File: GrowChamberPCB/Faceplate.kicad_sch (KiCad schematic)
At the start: 34 parts, among them J1 Conn_01x02_Pin, J10 Conn_01x02_Pin, J11 Conn_01x02_Pin, J12 Conn_01x03_Pin, J13 Conn_01x03_Pin, J14 Conn_01x03_Pin, J15 Conn_01x04_Pin, J2 Conn_01x03_Pin, J3 Conn_01x04_Pin, J4 Conn_01x02_Pin, J5 Conn_01x02_Pin, J6 Conn_01x02_Pin, J7 Conn_01x02_Pin, J8 Conn_01x02_Pin, J9 Conn_01x02_Pin, SW2 ResetButton_External, SW4 BootMode_External, U19 To Faceplate, U20 PCA9555APW,118

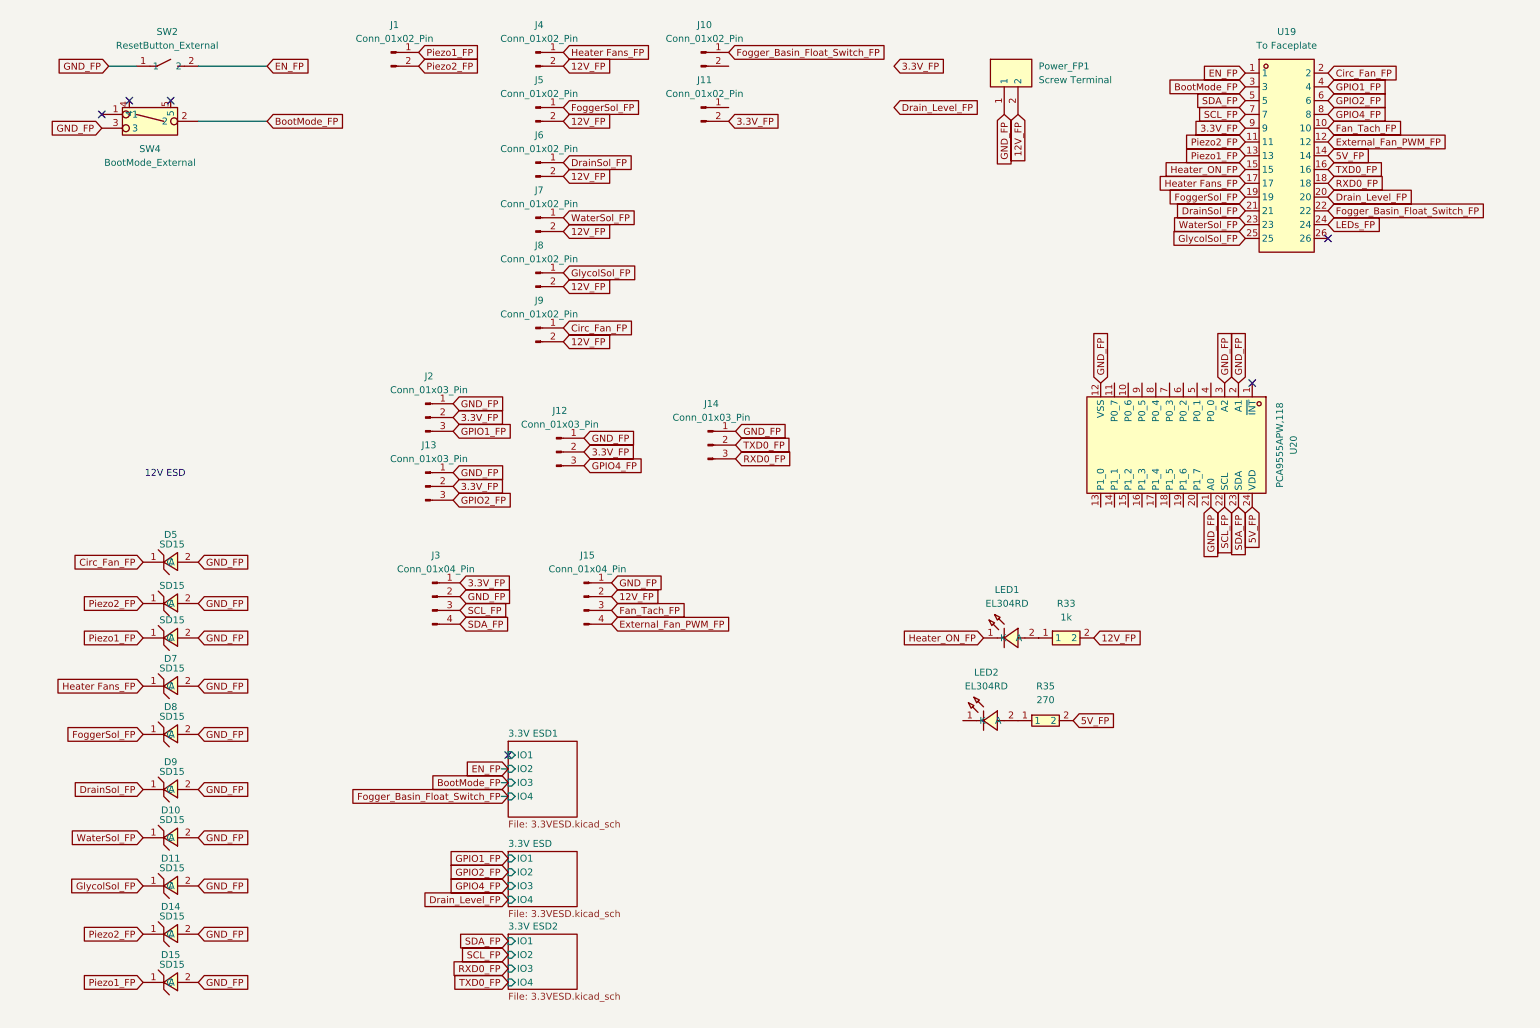
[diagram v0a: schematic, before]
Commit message: started PCB
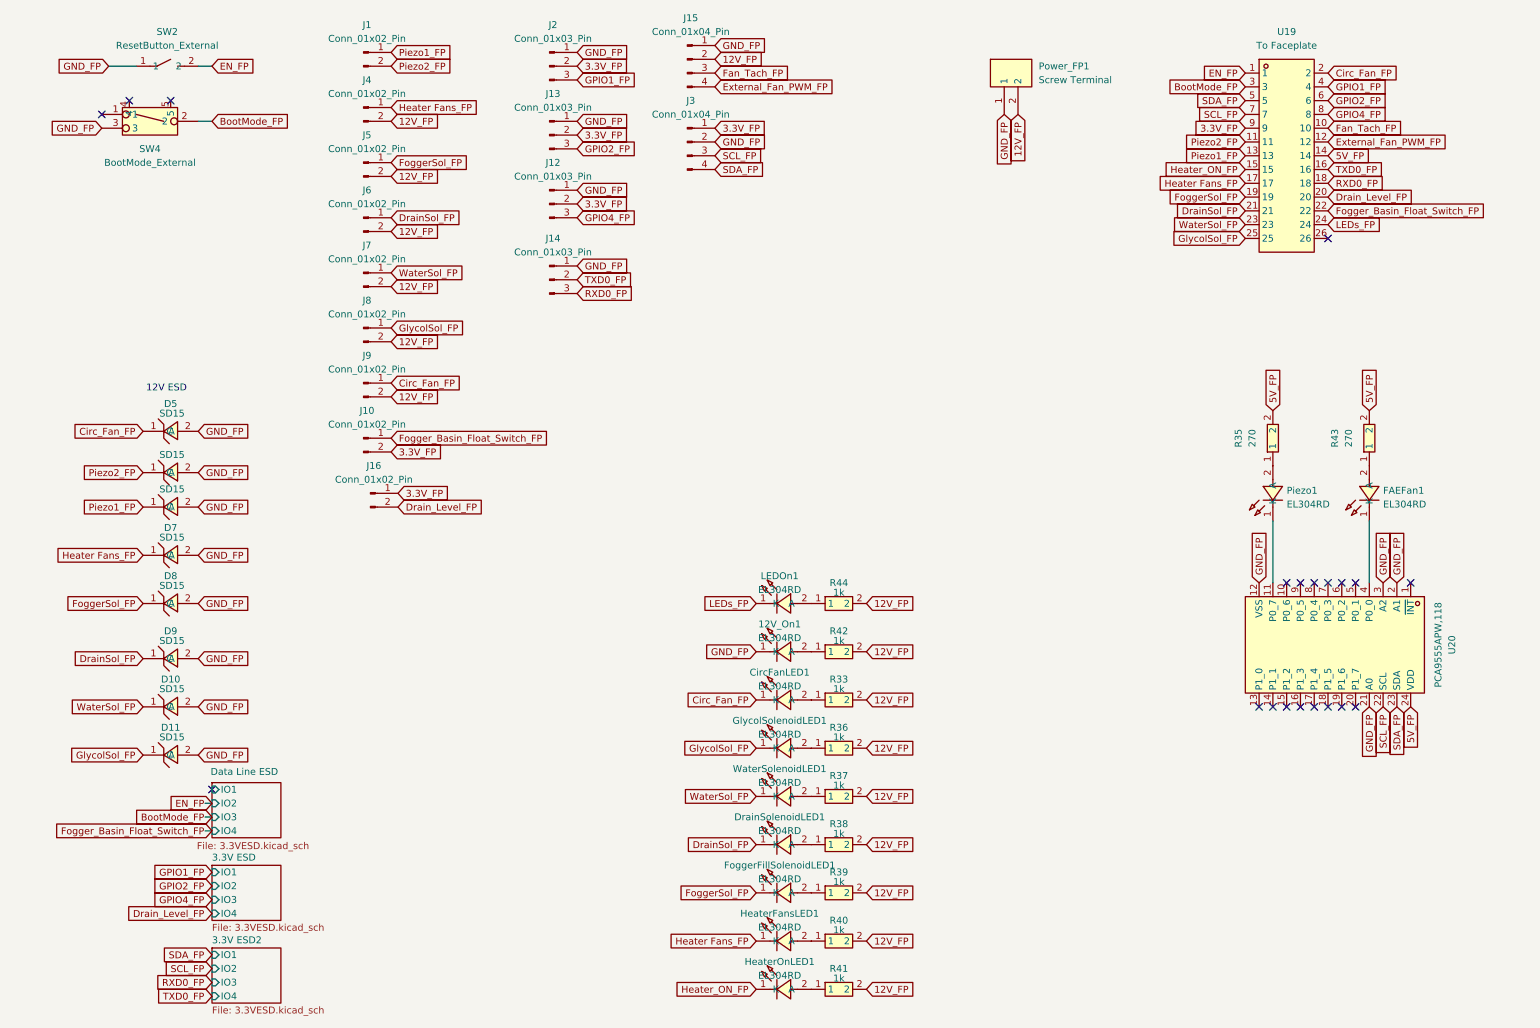
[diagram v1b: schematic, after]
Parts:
- removed D14, D15: SD15, easyeda2kicad:SOD-323_L1.7-W1.3-LS2.6-RD, symbol easyeda2kicad:SD15_C2931147
- removed J11: Conn_01x02_Pin, Connector_Molex:Molex_KK-254_AE-6410-02A_1x02_P2.54mm_Vertical, symbol Connector:Conn_01x02_Pin
- added 12V_On1, DrainSolenoidLED1, FAEFan1, FoggerFillSolenoidLED1, GlycolSolenoidLED1, HeaterFansLED1, HeaterOnLED1, LEDOn1, WaterSolenoidLED1: EL304RD, easyeda2kicad:LED-TH_BD3.9-P2.54-RD_RED, symbol easyeda2kicad:EL304RD
- added J16: Conn_01x02_Pin, Connector_Molex:Molex_KK-254_AE-6410-02A_1x02_P2.54mm_Vertical, symbol Connector:Conn_01x02_Pin
- added R36, R37, R38, R39, R40, R41, R42, R44: 1k, easyeda2kicad:R0603, symbol easyeda2kicad:FRC0603J102TS
- added R43: 270, easyeda2kicad:R0603, symbol easyeda2kicad:0603WAF2700T5E
- renumbered LED1 to CircFanLED1, LED2 to Piezo1
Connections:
- net 12V_FP: now also R36.2, R37.2, R38.2, R39.2, R40.2, R41.2, R42.2, R44.2
- net 3.3V_FP: now also J10.2 (Pin_2), J16.1 (Pin_1)
- net 5V_FP: now also R43.2
- net Circ_Fan_FP: now also CircFanLED1.1 (K)
- net DrainSol_FP: now also DrainSolenoidLED1.1 (K)
- net Drain_Level_FP: now also J16.2 (Pin_2)
- net FoggerSol_FP: now also FoggerFillSolenoidLED1.1 (K)
- net GND_FP: now also 12V_On1.1 (K)
- net GlycolSol_FP: now also GlycolSolenoidLED1.1 (K)
- net Heater Fans_FP: now also HeaterFansLED1.1 (K)
- net Heater_ON_FP: now also HeaterOnLED1.1 (K); no longer CircFanLED1.1 (K)
- net LEDs_FP: now also LEDOn1.1 (K)
- net WaterSol_FP: now also WaterSolenoidLED1.1 (K)
- net at U20.11 (P0_7): now also Piezo1.1 (K)
- net at U20.4 (P0_0): now also FAEFan1.1 (K)
- new net: 12V_On1.2 (A), R42.1
- new net: GlycolSolenoidLED1.2 (A), R36.1
- new net: HeaterOnLED1.2 (A), R41.1
- new net: FAEFan1.2 (A), R43.1
- new net: R37.1, WaterSolenoidLED1.2 (A)
- new net: DrainSolenoidLED1.2 (A), R38.1
- new net: FoggerFillSolenoidLED1.2 (A), R39.1
- new net: HeaterFansLED1.2 (A), R40.1
- new net: LEDOn1.2 (A), R44.1
- no-connect marks 6 -> 20
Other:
- sheet 3.3V ESD1 renamed Data Line ESD
- moved on the sheet: CircFanLED1, D10, D11, D5, D7, D8, D9, J1, J10, J12, J13, J14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
